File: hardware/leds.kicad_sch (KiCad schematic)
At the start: 123 parts

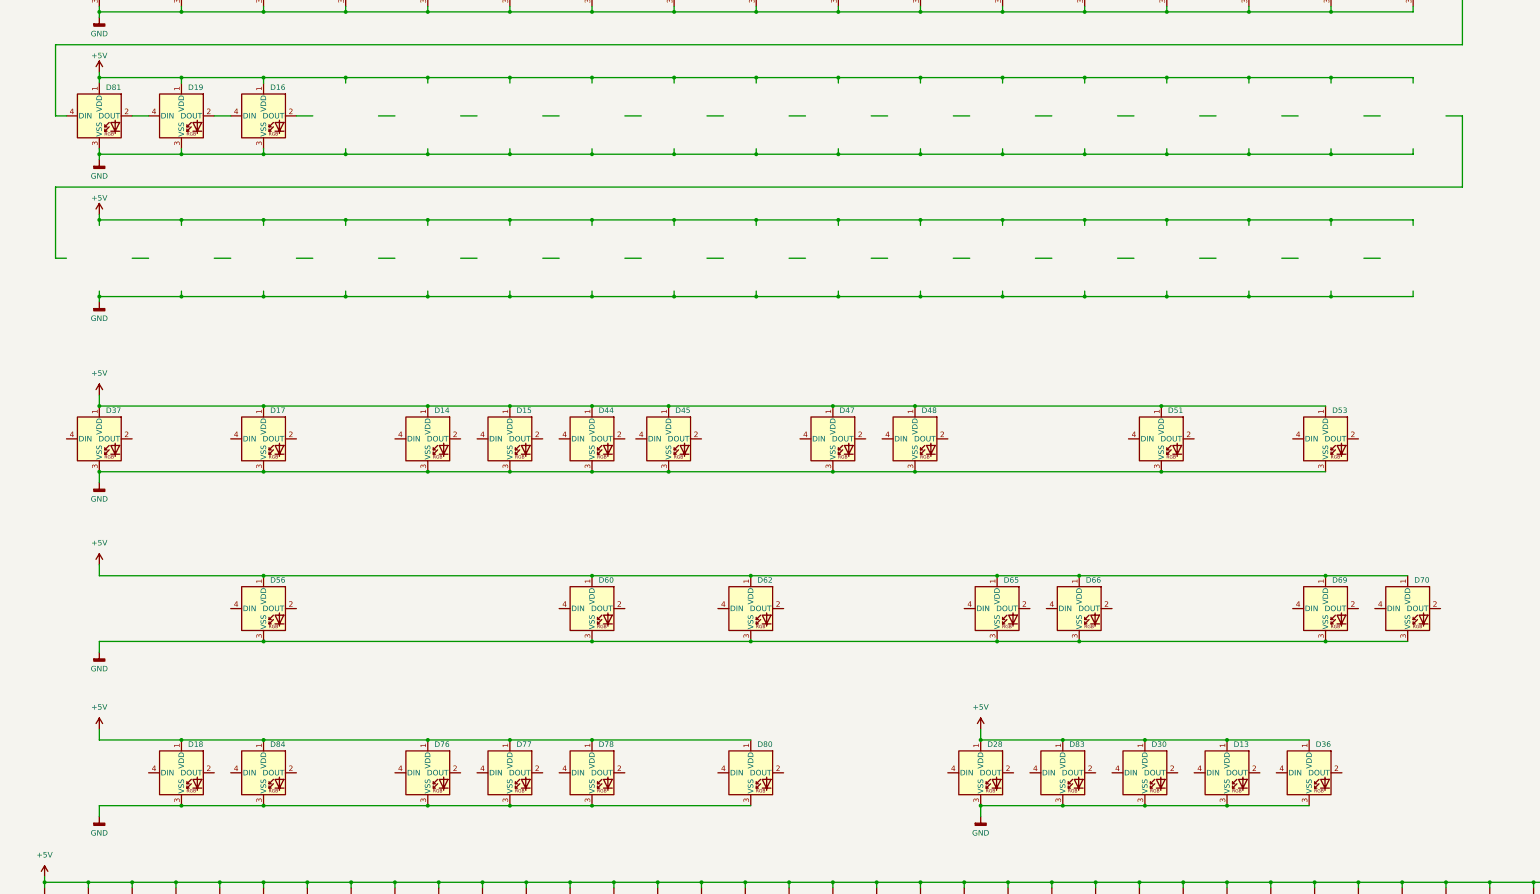
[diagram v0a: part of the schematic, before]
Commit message: Initial routing done
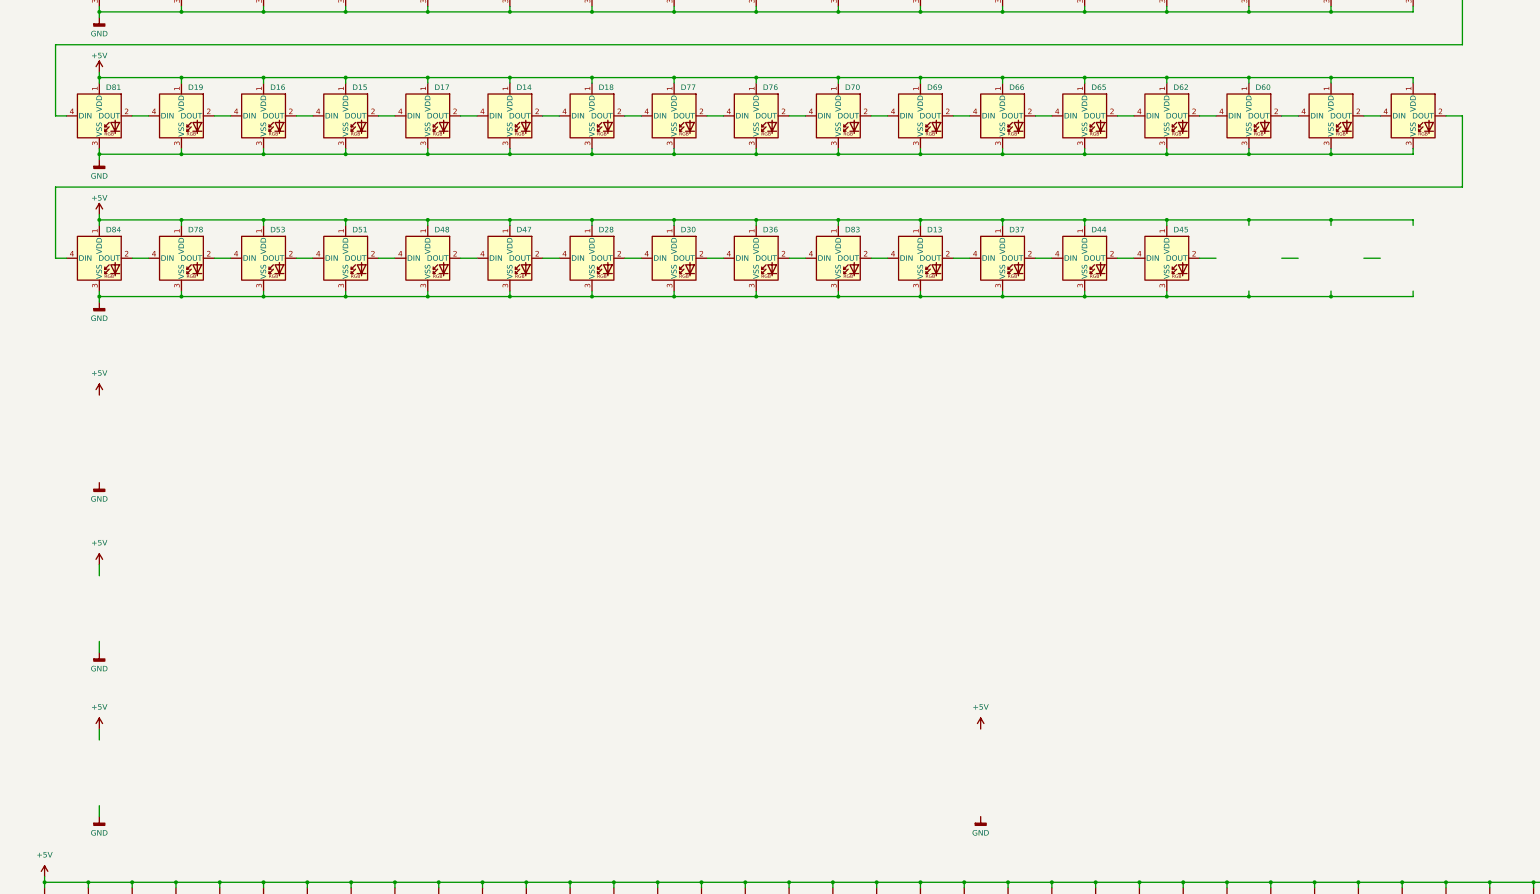
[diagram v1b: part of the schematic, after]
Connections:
- net at D76.2 (DOUT): now also D70.4 (DIN)
- net at D76.4 (DIN): now also D77.2 (DOUT)
- net at D28.2 (DOUT): now also D30.4 (DIN)
- net at D28.4 (DIN): now also D47.2 (DOUT)
- net at D53.2 (DOUT): now also D51.4 (DIN)
- net at D53.4 (DIN): now also D78.2 (DOUT)
- net at D18.2 (DOUT): now also D77.4 (DIN)
- net at D18.4 (DIN): now also D14.2 (DOUT)
- net at D48.2 (DOUT): now also D47.4 (DIN)
- net at D48.4 (DIN): now also D51.2 (DOUT)
- net at D15.2 (DOUT): now also D17.4 (DIN)
- net at D15.4 (DIN): now also D16.2 (DOUT)
- net at D80.2 (DOUT): now also D56.4 (DIN)
- net at D80.4 (DIN): now also D60.2 (DOUT)
- net at D17.2 (DOUT): now also D14.4 (DIN)
- net at D30.2 (DOUT): now also D36.4 (DIN)
- net at D44.2 (DOUT): now also D45.4 (DIN)
- net at D44.4 (DIN): now also D37.2 (DOUT)
- net at D83.2 (DOUT): now also D13.4 (DIN)
- net at D83.4 (DIN): now also D36.2 (DOUT)
- net at D62.2 (DOUT): now also D60.4 (DIN)
- net at D62.4 (DIN): now also D65.2 (DOUT)
- net at D66.2 (DOUT): now also D65.4 (DIN)
- net at D66.4 (DIN): now also D69.2 (DOUT)
- net at D56.2 (DOUT): now also D84.4 (DIN)
- net at D13.2 (DOUT): now also D37.4 (DIN)
- net at D69.4 (DIN): now also D70.2 (DOUT)
- net at D84.2 (DOUT): now also D78.4 (DIN)
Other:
- moved on the sheet: D13, D14, D15, D17, D18, D28, D30, D36, D37, D44, D45, D47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
